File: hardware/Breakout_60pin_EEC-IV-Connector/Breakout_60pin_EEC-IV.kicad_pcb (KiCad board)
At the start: 2 copper layers, 139.7 x 62.2 mm, 17 parts, among them J1 Conn_01x01, J10 Conn_01x10, J11 Conn_01x10, J12 Conn_01x10, J13 Conn_01x10, J14 EEC-IV, J2 Conn_01x10, J3 Conn_01x10, J4 Conn_01x10, J5 Conn_01x10, J6 Conn_01x10, J7 Conn_01x10, J8 Conn_01x10, J9 Conn_01x10

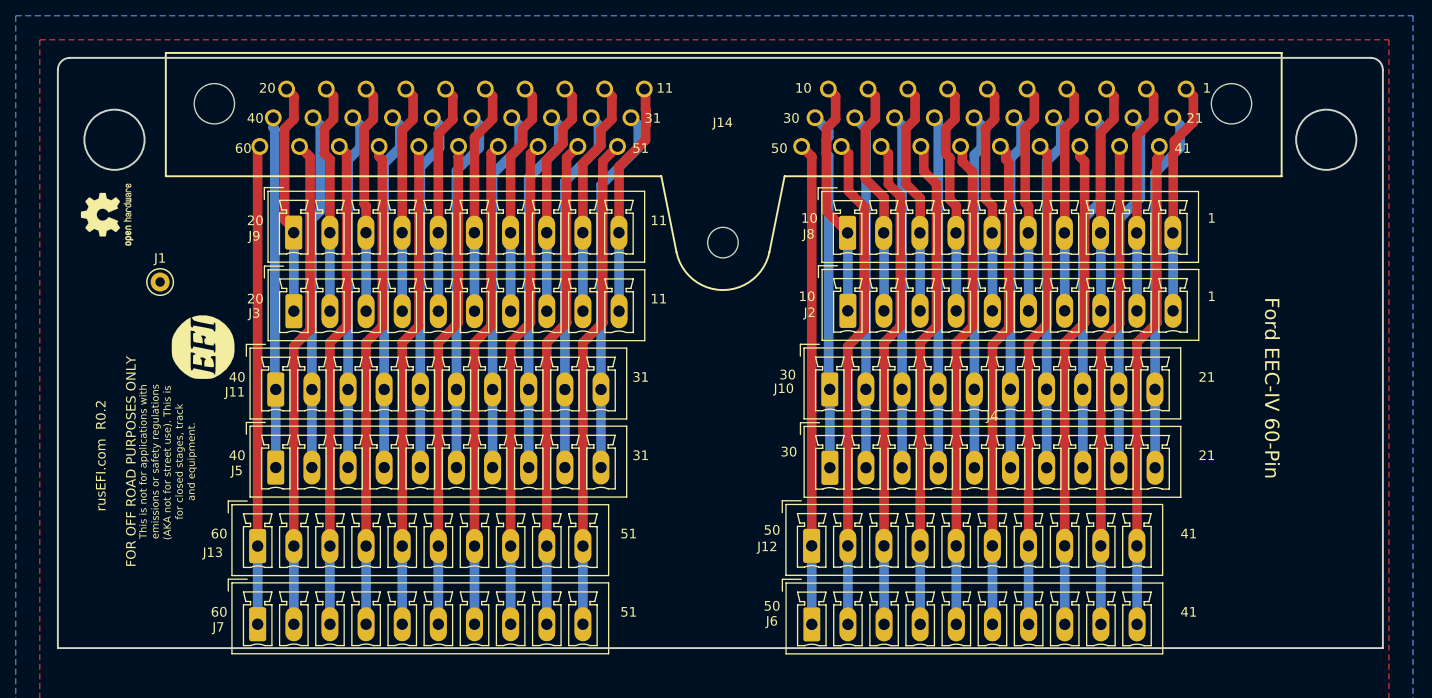
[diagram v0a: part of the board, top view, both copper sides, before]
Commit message: update pcb files
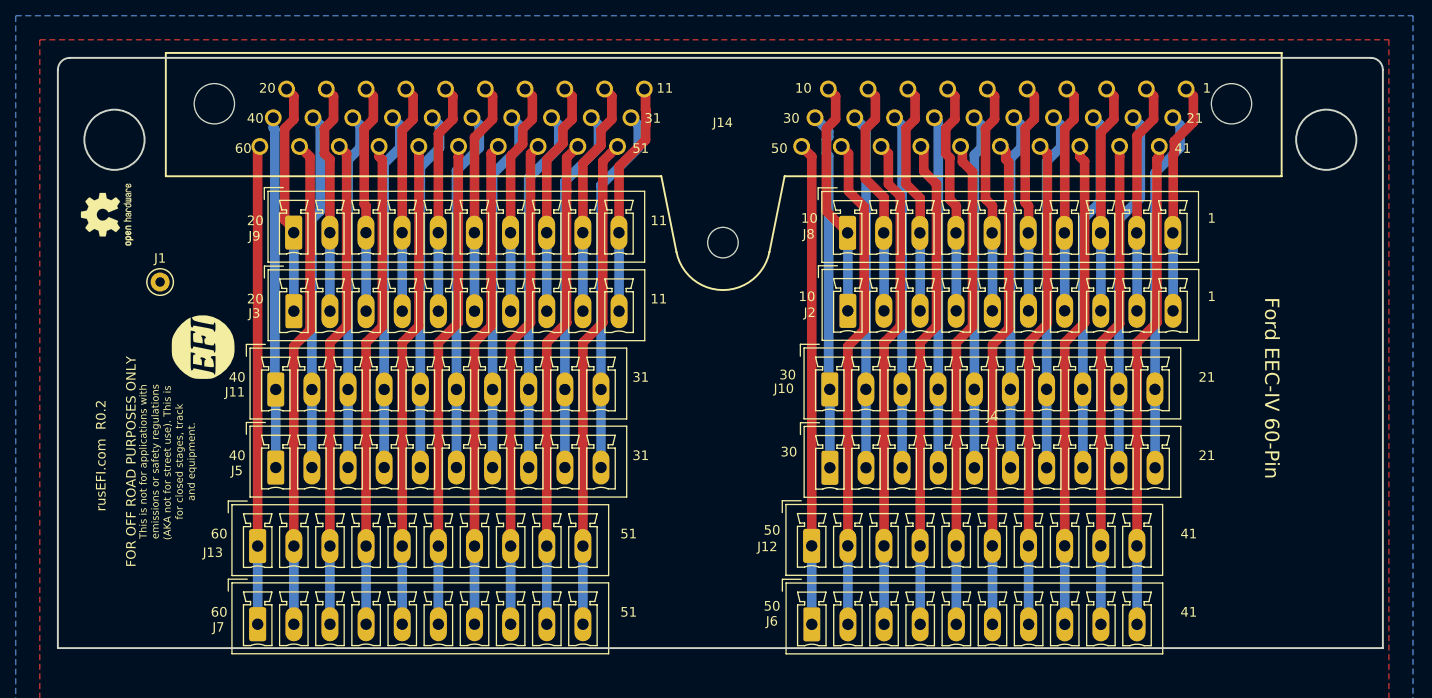
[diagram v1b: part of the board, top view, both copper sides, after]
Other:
- net class Default removed
- net class traces_50_mils removed
